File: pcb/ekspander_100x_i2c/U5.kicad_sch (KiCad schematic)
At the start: 5 parts, among them J12 DG127A-5.08-06P-14-00AH, J13 DG127A-5.08-06P-14-00AH, J14 DG127A-5.08-06P-14-00AH, U5 MCP23017_SP

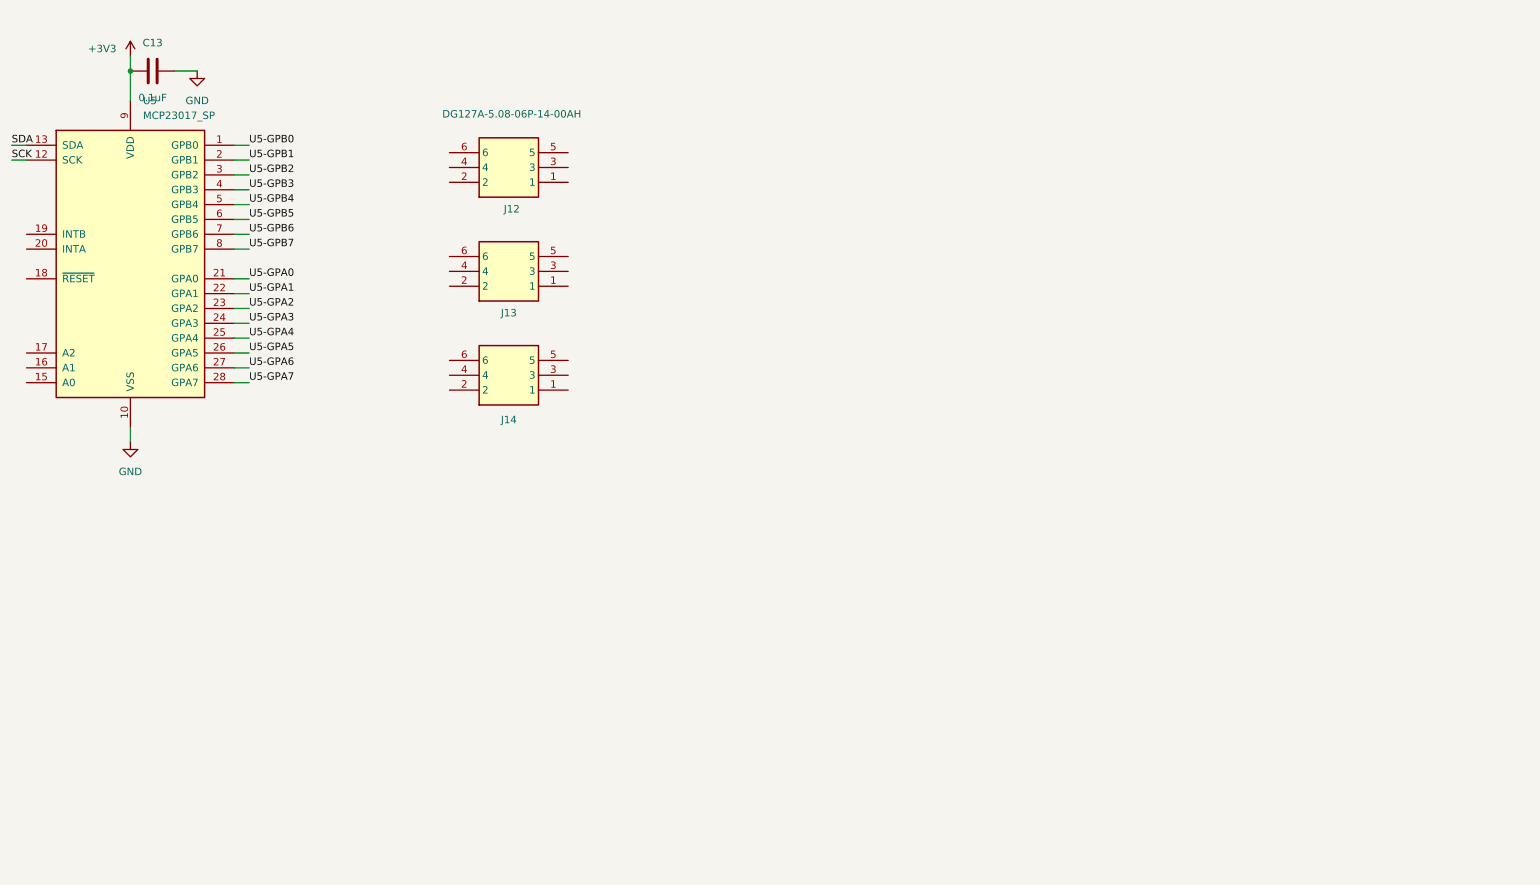
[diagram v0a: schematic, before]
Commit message: Ekspander U5 - U6 update
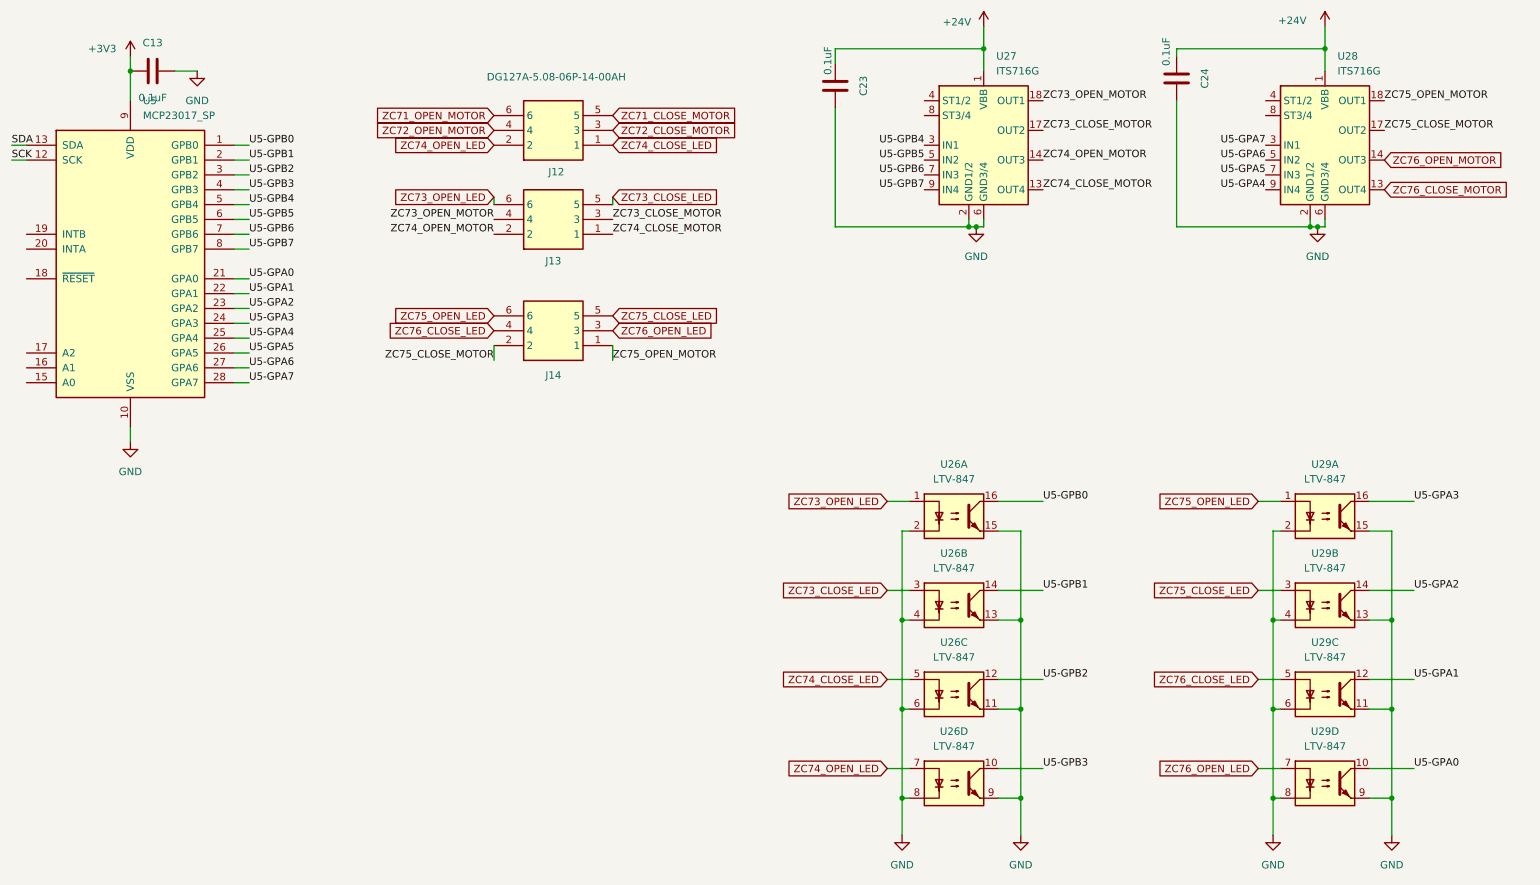
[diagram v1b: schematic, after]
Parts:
- added C23, C24: 0.1uF, Capacitor_SMD:C_0805_2012Metric_Pad1.18x1.45mm_HandSolder, symbol Device:C
- added U26, U29: LTV-847, Package_DIP:DIP-16_W7.62mm, symbol Isolator:LTV-847
- added U27, U28: ITS716G, Package_SO:SOIC-20W_7.5x12.8mm_P1.27mm, symbol Driver_FET:ITS716G
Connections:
- net GND: now also C23.2, C24.2, U26.11, U26.13, U26.15, U26.2, U26.4, U26.6, U26.8, U26.9, U27.2 (GND1/2), U27.6 (GND3/4), U28.2 (GND1/2), U28.6 (GND3/4), U29.11, U29.13, U29.15, U29.2, U29.4, U29.6, U29.8, U29.9
- net U5-GPA0: now also U29.10
- net U5-GPA1: now also U29.12
- net U5-GPA2: now also U29.14
- net U5-GPA3: now also U29.16
- net U5-GPA4: now also U28.9 (IN4)
- net U5-GPA5: now also U28.7 (IN3)
- net U5-GPA6: now also U28.5 (IN2)
- net U5-GPA7: now also U28.3 (IN1)
- net U5-GPB0: now also U26.16
- net U5-GPB1: now also U26.14
- net U5-GPB2: now also U26.12
- net U5-GPB3: now also U26.10
- net U5-GPB4: now also U27.3 (IN1)
- net U5-GPB5: now also U27.5 (IN2)
- net U5-GPB6: now also U27.7 (IN3)
- net U5-GPB7: now also U27.9 (IN4)
- net ZC74_CLOSE_LED: now reaches J12.1
- net ZC74_CLOSE_LED: now also U26.5
- net ZC74_OPEN_LED: now reaches J12.2
- net ZC74_OPEN_LED: now also U26.7
- net ZC72_CLOSE_MOTOR: now reaches J12.3
- net ZC72_OPEN_MOTOR: now reaches J12.4
- net ZC71_CLOSE_MOTOR: now reaches J12.5
- net ZC71_OPEN_MOTOR: now reaches J12.6
- net ZC75_OPEN_MOTOR: now reaches J14.1
- net ZC75_OPEN_MOTOR: now also U28.18 (OUT1)
- net ZC75_CLOSE_MOTOR: now reaches J14.2
- net ZC75_CLOSE_MOTOR: now also U28.17 (OUT2)
- net ZC76_OPEN_LED: now reaches J14.3
- net ZC76_OPEN_LED: now also U29.7
- net ZC76_CLOSE_LED: now reaches J14.4
- net ZC76_CLOSE_LED: now also U29.5
- net ZC75_CLOSE_LED: now reaches J14.5
- net ZC75_CLOSE_LED: now also U29.3
- net ZC75_OPEN_LED: now reaches J14.6
- net ZC75_OPEN_LED: now also U29.1
- net ZC74_CLOSE_MOTOR: now reaches J13.1
- net ZC74_CLOSE_MOTOR: now also U27.13 (OUT4)
- net ZC74_OPEN_MOTOR: now reaches J13.2
- net ZC74_OPEN_MOTOR: now also U27.14 (OUT3)
- net ZC73_CLOSE_MOTOR: now reaches J13.3
- net ZC73_CLOSE_MOTOR: now also U27.17 (OUT2)
- net ZC73_OPEN_MOTOR: now reaches J13.4
- net ZC73_OPEN_MOTOR: now also U27.18 (OUT1)
- net ZC73_CLOSE_LED: now reaches J13.5
- net ZC73_CLOSE_LED: now also U26.3
- net ZC73_OPEN_LED: now reaches J13.6
- net ZC73_OPEN_LED: now also U26.1
- new net +24V: C23.1, C24.1, U27.1 (VBB), U27.10 (VBB), U27.11 (VBB), U27.12 (VBB), U27.15 (VBB), U27.16 (VBB), U27.19 (VBB), U27.20 (VBB), U28.1 (VBB), U28.10 (VBB), U28.11 (VBB), U28.12 (VBB), U28.15 (VBB), U28.16 (VBB), U28.19 (VBB), U28.20 (VBB)
- new net ZC76_CLOSE_MOTOR: U28.13 (OUT4)
- new net ZC76_OPEN_MOTOR: U28.14 (OUT3)
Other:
- moved on the sheet: J12, J13, J14
